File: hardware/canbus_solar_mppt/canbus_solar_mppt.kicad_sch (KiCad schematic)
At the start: 19 parts

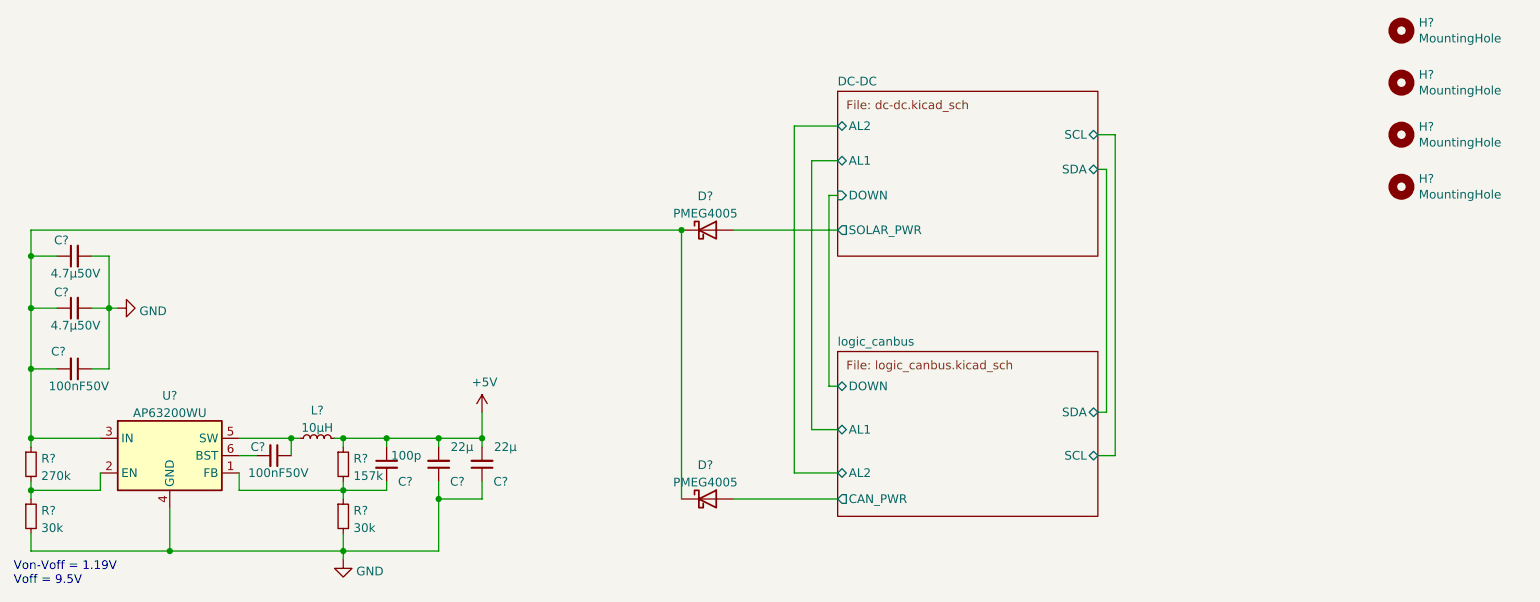
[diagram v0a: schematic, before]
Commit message: WIP: complete DC/DC engine
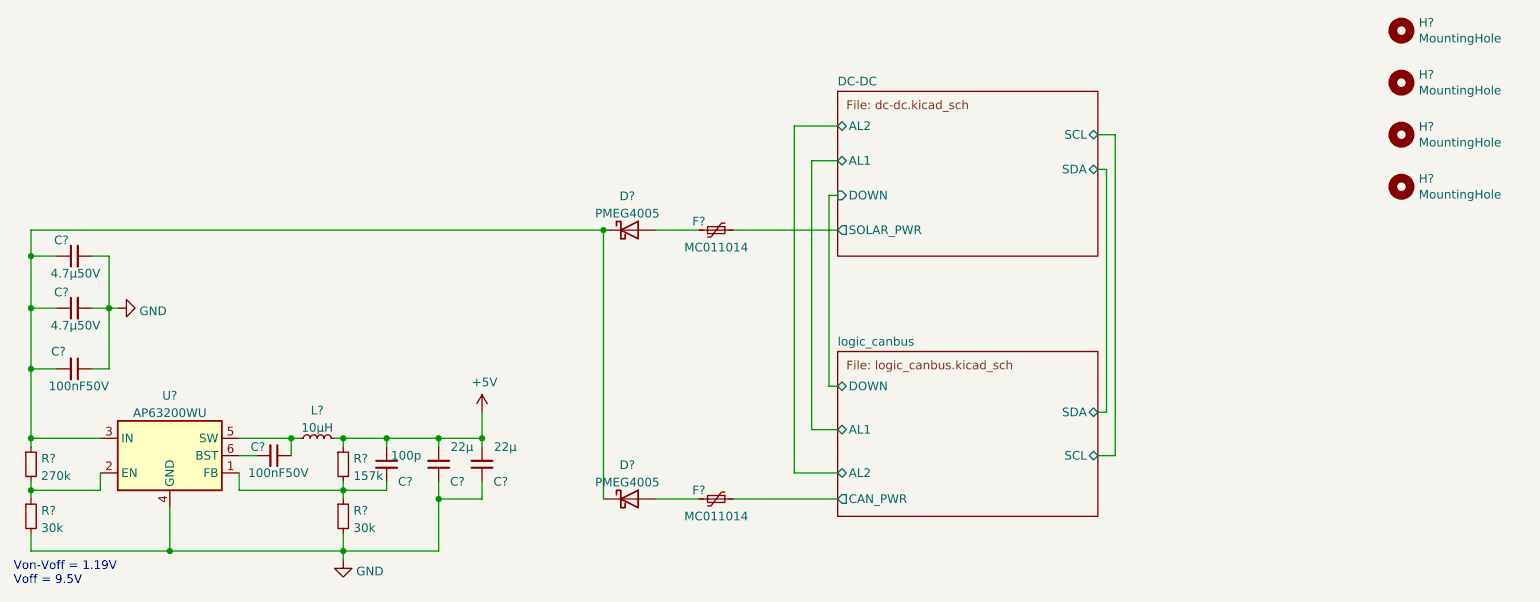
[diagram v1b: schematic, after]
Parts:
- added F? (x2): MC011014, Fuse:Fuse_2920_7451Metric_Pad2.10x5.45mm_HandSolder, symbol Device:Polyfuse_Small
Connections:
- net DC-DC/SOLAR_PWR: now also F?.1; no longer D?.2 (A)
- net logic_canbus/CAN_PWR: now also F?.1; no longer D?.2 (A)
- new net: D?.2 (A), F?.2 (x2)
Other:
- moved on the sheet: D?
